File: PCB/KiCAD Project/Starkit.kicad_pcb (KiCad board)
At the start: 2 copper layers, 65 x 112.5 mm, 34 parts, among them J1 Screw_Terminal_01x02, J11 Conn_01x06_Pin, J2 Screw_Terminal_01x02, J3 Screw_Terminal_01x02, J4 Screw_Terminal_01x02, J5 Conn_01x02, J6 Conn_01x02, U4 ESP32-DEVKITC-32D, X1 Conn_01x03_Pin, X2 Conn_01x03_Pin, Y1 Conn_01x03_Pin, Y2 Conn_01x03_Pin

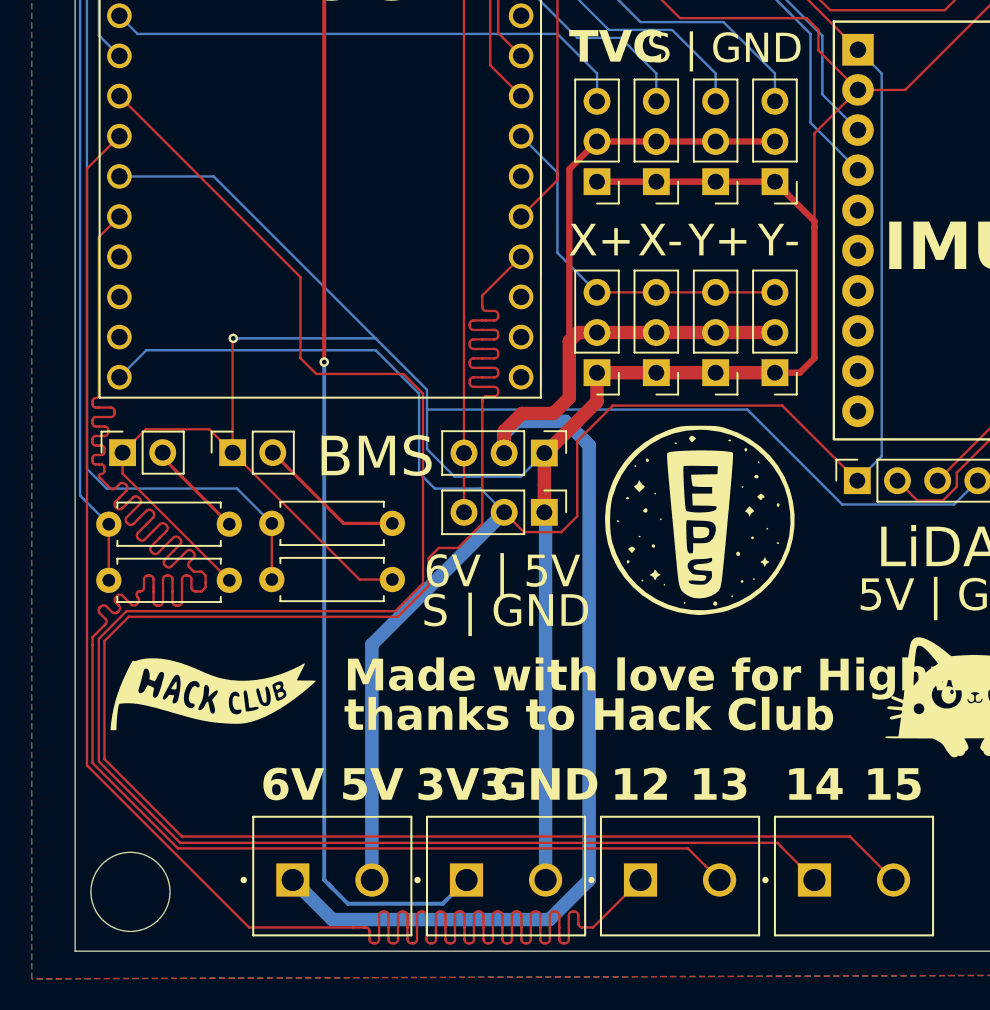
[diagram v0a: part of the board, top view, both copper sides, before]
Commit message: 23-06-2025
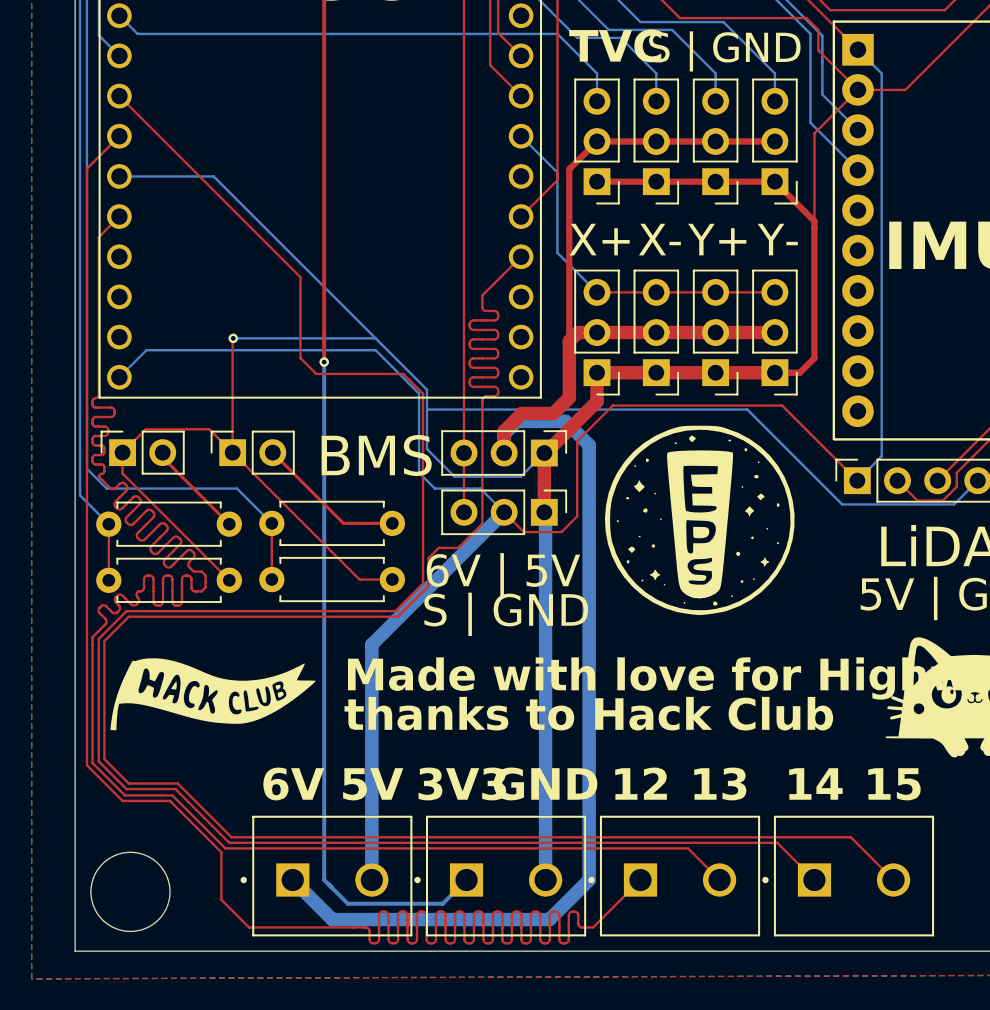
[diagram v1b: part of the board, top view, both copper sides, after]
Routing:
- net /12: track 119.9 -> 121.7 mm

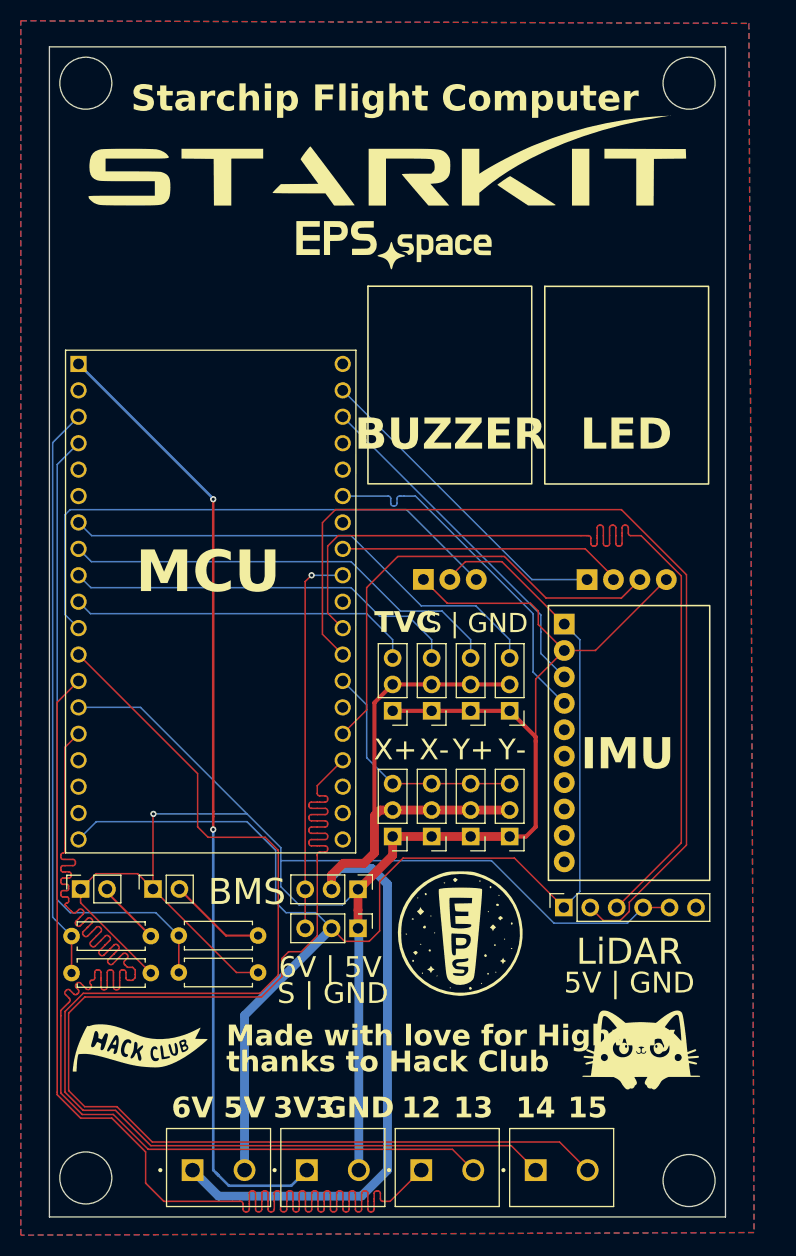
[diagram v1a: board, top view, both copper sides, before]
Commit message: 09-07-2025
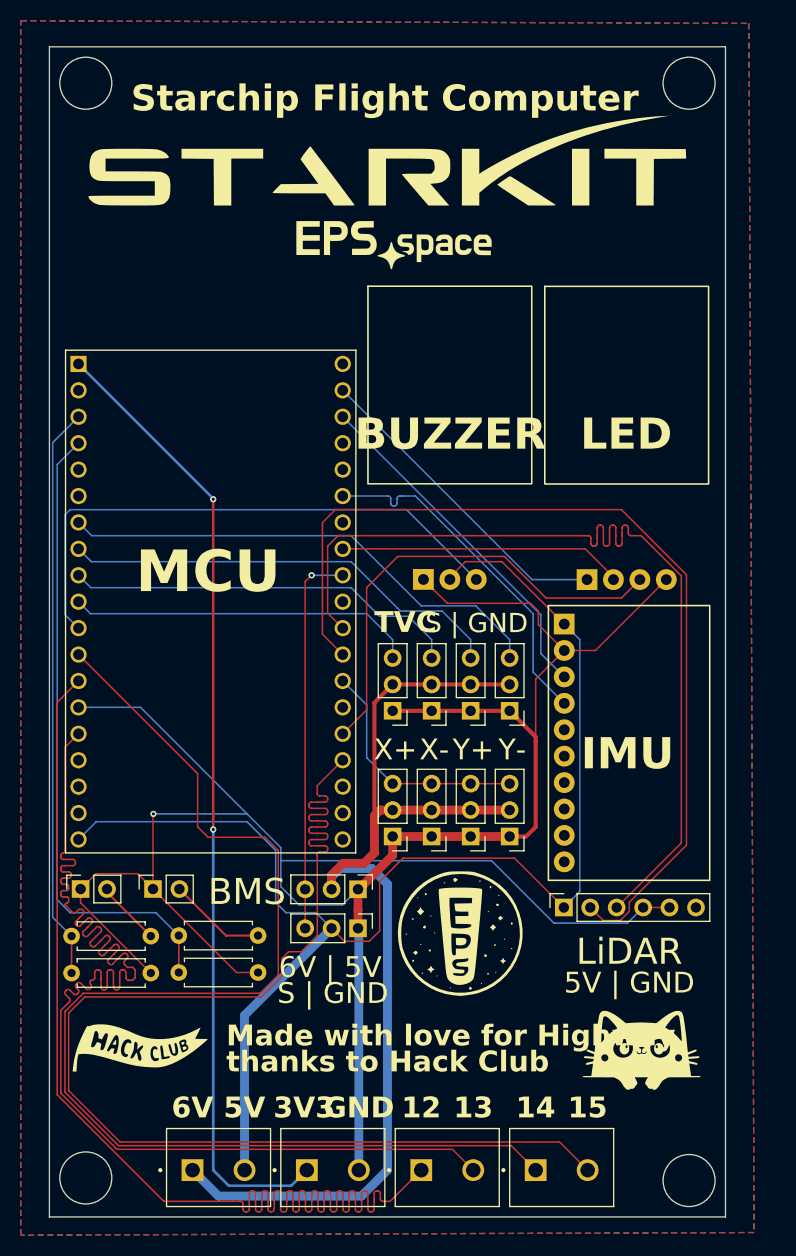
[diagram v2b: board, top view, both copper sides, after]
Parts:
- removed the G*** at (174.4, 132.8)
- added G***: LOGO, Starchip:Cat, F.Cu at (174.4, 132.8)
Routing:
- net /12: track 121.7 -> 119.9 mm
